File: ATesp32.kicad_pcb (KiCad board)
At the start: 4 copper layers, 18 x 51.2 mm, 51 parts, among them J1 USB_C_Receptacle_USB2.0_16P, J2 JST PH, Q1 DMP2045U, SW1 SW_Push, SW2 SW_Push, U1 ESP32-S3, U2 ATmega32A-P, U3 MCP73831-2-OT, U4 AP2112K-3.3, U5 CP2102N-Axx-xQFN24, Y1 40 MHz

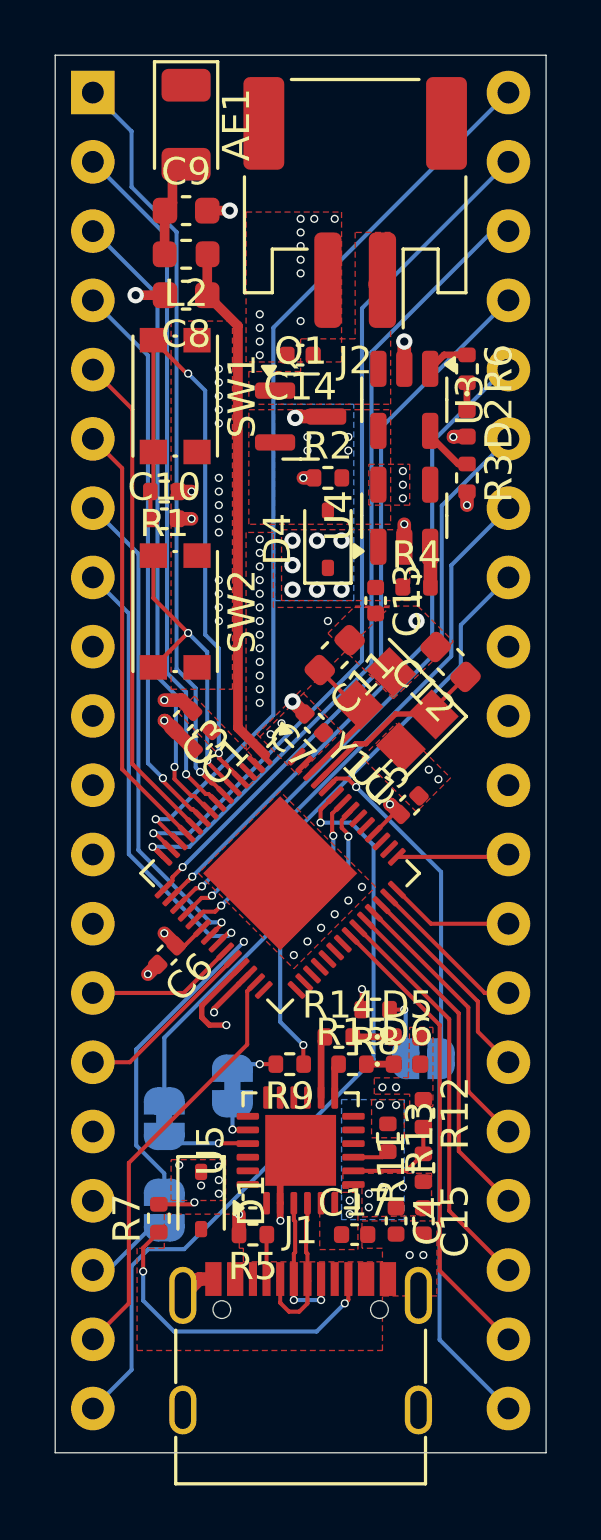
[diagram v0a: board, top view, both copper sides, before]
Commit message: cleanup
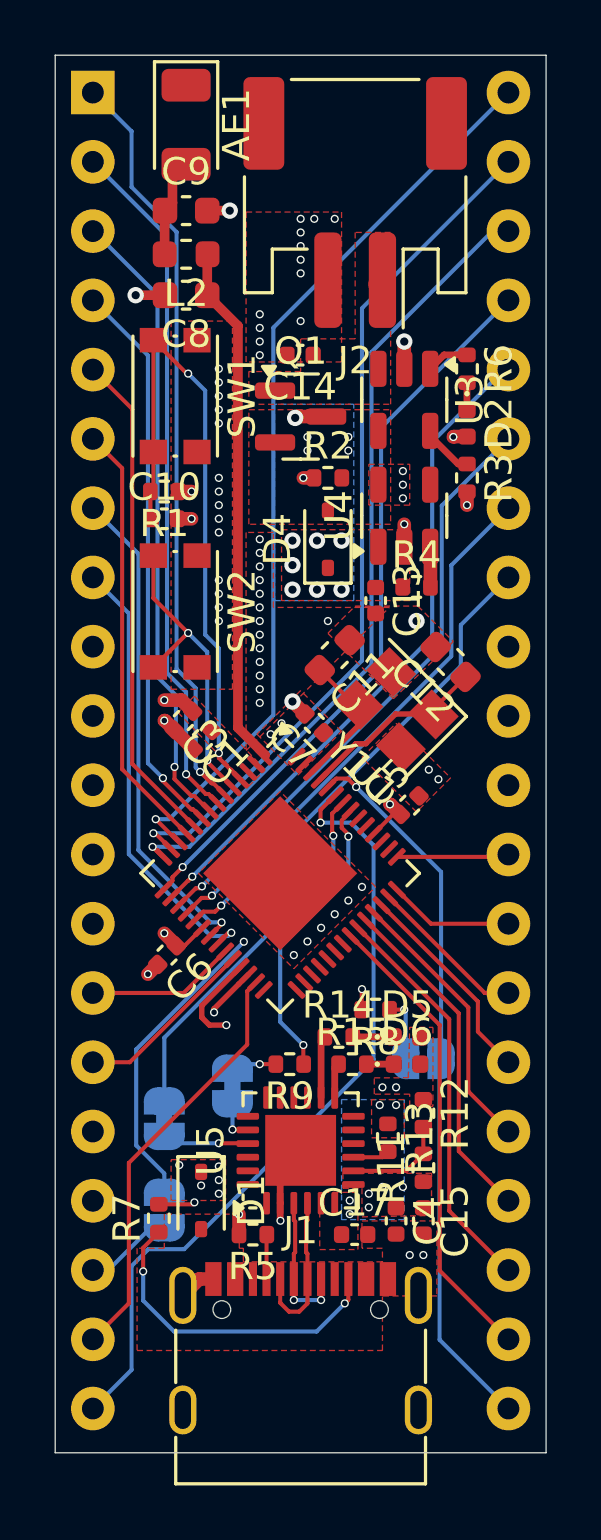
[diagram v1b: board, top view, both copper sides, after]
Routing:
- net GND: track 15.4 -> 14.3 mm
- net PD4: track 3.26 -> 2.19 mm
- net PA2: track 29.7 -> 29.1 mm
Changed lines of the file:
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@@
 	)
 	(segment
-		(start 79.0125 55.7125)
-		(end 79.025 55.7)
-		(width 0.355542)
-		(layer "F.Cu")
-		(net 1)
-	)
-	(segment
 		(start 79.8 54)
 		(end 79.3 54.5)
@@
 	)
 	(segment
-		(start 83.25 90.9125)
-		(end 84 90.1625)
-		(width 0.25)
-		(layer "F.Cu")
-		(net 3)
-	)
-	(segment
 		(start 83.25 92.1)
 		(end 83.25 92.732108)
@@
 	)
 	(segment
-		(start 80.5 55.775)
-		(end 80.525 55.75)
-		(width 0.355542)
-		(layer "F.Cu")
-		(net 3)
-	)
-	(segment
 		(start 80.28 94.88)
 		(end 79.68 95.48)
@@
 	)
 	(segment
-		(start 87.390488 77.839411)
-		(end 87.660589 77.839411)
-		(width 0.15)
-		(layer "F.Cu")
-		(net 5)
-	)
-	(segment
-		(start 79.439411 82.639411)
-		(end 79.439411 82.660589)
-		(width 0.5)
-		(layer "F.Cu")
-		(net 5)
-	)
-	(segment
 		(start 80.039411 74.060589)
 		(end 79.628822 73.65)
@@
 	)
 	(segment
-		(start 80.575 57.3125)
-		(end 80.5875 57.3)
-		(width 0.355542)
-		(layer "F.Cu")
-		(net 7)
-	)
-	(segment
 		(start 80.575 58.8)
 		(end 81.7 59.925)
@@
 	)
 	(segment
-		(start 78.6 65.890001)
-		(end 78.490001 66)
-		(width 0.15)
-		(layer "F.Cu")
-		(net 8)
-	)
-	(segment
-		(start 78.490001 66.970001)
-		(end 78.52 67)
-		(width 0.15)
-		(layer "F.Cu")
-		(net 8)
-	)
-	(segment
 		(start 78.6 60.45)
 		(end 78.6 64.55)
@@
 	)
 	(segment
-		(start 84.324991 94.954991)
-		(end 84.25 94.88)
-		(width 0.15)
-		(layer "F.Cu")
-		(net 16)
-	)
-	(segment
 		(start 84.25 93.949999)
 		(end 84.2 93.899999)
@@
 	)
 	(segment
-		(start 83.25 94.88)
-		(end 83.175 94.955)
-		(width 0.15)
-		(layer "F.Cu")
-		(net 16)
-	)
-	(segment
 		(start 84.25 95.775)
 		(end 84.25 94.88)
@@
 	)
 	(segment
-		(start 82.75 93.26)
-		(end 82.76 93.25)
-		(width 0.15)
-		(layer "F.Cu")
-		(net 18)
-	)
-	(segment
 		(start 82.75 94.88)
 		(end 82.75 93.26)
@@
 	)
 	(segment
-		(start 76.38 94.55)
-		(end 76.95 94.55)
-		(width 0.15)
-		(layer "B.Cu")
-		(net 21)
-	)
-	(segment
 		(start 76.95 94.55)
 		(end 78.5 93)
@@
 	)
 	(segment
-		(start 78.5 93)
-		(end 79 93)
-		(width 0.15)
-		(layer "B.Cu")
-		(net 21)
-	)
-	(segment
 		(start 78.6 69.9125)
 		(end 78.6 68.35)
@@
 		(net 26)
 	)
-	(segment
-		(start 82.05 89.9)
-		(end 82.0625 89.9125)
-		(width 0.15)
-		(layer "F.Cu")
-		(net 26)
-	)
 	(via
 		(at 81 89.9)
@@
 	)
 	(segment
-		(start 79.25 89.9)
-		(end 79 89.65)
-		(width 0.15)
-		(layer "B.Cu")
-		(net 26)
-	)
-	(segment
 		(start 81 89.9)
 		(end 79.25 89.9)
@@
 	)
 	(segment
-		(start 81.65 87)
-		(end 81.5 87.15)
-		(width 0.15)
-		(layer "B.Cu")
-		(net 27)
-	)
-	(segment
 		(start 81.5 89.4)
 		(end 82.05 89.4)
@@
 		(net 28)
 	)
-	(segment
-		(start 82.05 89.4)
-		(end 82.0625 89.4125)
-		(width 0.15)
-		(layer "F.Cu")
-		(net 28)
-	)
 	(via
 		(at 81.5 89.4)
@@
 	)
 	(segment
-		(start 88.75 63.963172)
-		(end 88.75 63.775)
-		(width 0.25)
-		(layer "F.Cu")
-		(net 29)
-	)
-	(segment
 		(start 88.76 69.5)
 		(end 88.76 68.035)
@@
 	)
 	(segment
-		(start 88.76 68.035)
-		(end 88.75 68.025)
-		(width 0.5)
-		(layer "F.Cu")
-		(net 30)
-	)
-	(segment
 		(start 85.50496 78.330518)
 		(end 85.50496 78.063238)
@@
 	)
 	(segment
-		(start 84.1 86.99)
-		(end 84.11 87)
-		(width 0.15)
-		(layer "F.Cu")
-		(net 31)
-	)
-	(segment
 		(start 85.75 78.575558)
 		(end 85.50496 78.330518)
@@
 	)
 	(segment
-		(start 85.83094 77.737258)
-		(end 85.83094 77.701903)
-		(width 0.15)
-		(layer "F.Cu")
-		(net 31)
-	)
-	(segment
 		(start 84.1 86.3)
 		(end 84.1 86.99)
@@
 	)
 	(segment
-		(start 84.75 86.14)
-		(end 84.89 86)
-		(width 0.25)
-		(layer "F.Cu")
-		(net 34)
-	)
-	(segment
 		(start 84.75 88.225)
 		(end 84.75 86.14)
@@
 	)
 	(segment
-		(start 85.25 87.14)
-		(end 85.39 87)
-		(width 0.25)
-		(layer "F.Cu")
-		(net 35)
-	)
-	(segment
 		(start 85.25 88.225)
 		(end 85.25 87.14)
@@
 	)
 	(segment
-		(start 78.972004 79.398959)
-		(end 78.936647 79.398959)
-		(width 0.15)
-		(layer "F.Cu")
-		(net 36)
-	)
-	(segment
 		(start 78.936647 79.398959)
 		(end 78.568844 79.031156)
@@
 	)
 	(segment
-		(start 91.036827 56.45)
-		(end 91.62 56.45)
-		(width 0.15)
-		(layer "B.Cu")
-		(net 36)
-	)
-	(segment
 		(start 86.6 72.349098)
 		(end 86.6 60.886827)
@@
 	)
 	(segment
-		(start 80.636898 77.701903)
-		(end 80.66906 77.701903)
-		(width 0.15)
-		(layer "F.Cu")
-		(net 38)
-	)
-	(segment
 		(start 79.990524 77.161596)
 		(end 80.096591 77.161596)
@@
 	)
 	(segment
-		(start 76.413173 56.45)
-		(end 76.38 56.45)
-		(width 0.15)
-		(layer "B.Cu")
-		(net 38)
-	)
-	(segment
 		(start 78.75 72.798959)
 		(end 78.75 58.786827)
@@
 	)
 	(segment
-		(start 91.531041 79.398959)
-		(end 91.62 79.31)
-		(width 0.15)
-		(layer "F.Cu")
-		(net 43)
-	)
-	(segment
 		(start 78.670867 78.532137)
 		(end 79.254847 79.116117)
@@
 	)
 	(segment
-		(start 91.62 61.53)
-		(end 91.468959 61.53)
-		(width 0.15)
-		(layer "B.Cu")
-		(net 46)
-	)
-	(segment
 		(start 91.468959 61.53)
 		(end 88.825 64.173959)
@@
 	)
 	(segment
-		(start 76.38 89.380228)
-		(end 76.38 89.47)
-		(width 0.15)
-		(layer "B.Cu")
-		(net 69)
-	)
-	(segment
-		(start 79.502334 78.833274)
-		(end 79.537689 78.833274)
-		(width 0.15)
-		(layer "F.Cu")
-		(net 70)
-	)
-	(segment
 		(start 78.68453 78.01547)
 		(end 79.502334 78.833274)
@@
 	)
 	(segment
-		(start 85.977207 73.823223)
-		(end 86.121142 73.823223)
-		(width 0.15)
-		(layer "F.Cu")
-		(net 92)
-	)
-	(segment
 		(start 88.8617 74.159619)
 		(end 87.4818 74.159619)
@@
 	)
 	(segment
-		(start 88.878858 73.967158)
-		(end 88.878858 74.176777)
-		(width 0.15)
-		(layer "F.Cu")
-		(net 93)
-	)
-	(segment
 		(start 86.020101 75.25)
 		(end 84.699569 76.570532)
 		(width 0.2)
 		(layer "F.Cu")
-		(net 93)
-	)
-	(segment
-		(start 88.878858 74.176777)
-		(end 88.8617 74.159619)
-		(width 0.2)
-		(layer "F.Cu")

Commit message: fix silk
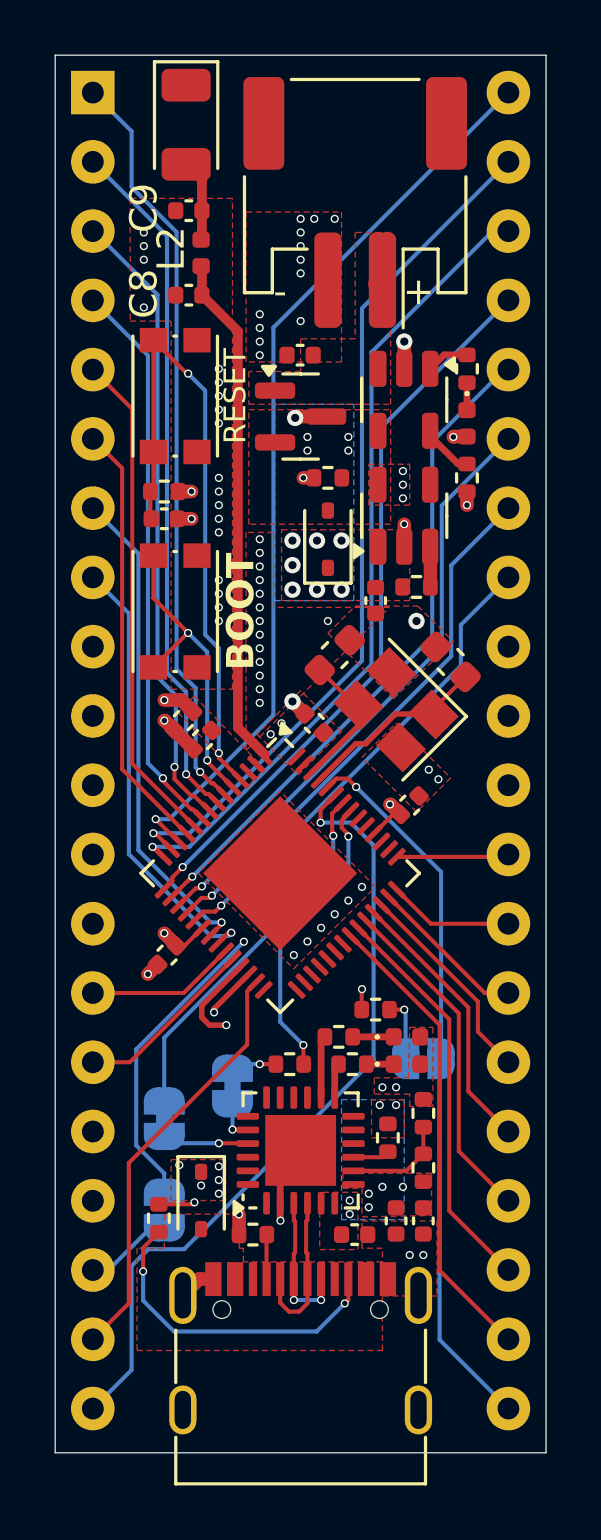
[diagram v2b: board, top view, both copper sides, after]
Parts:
- C8, C9: footprint Capacitor_SMD:C_0603_1608Metric -> Capacitor_SMD:C_0402_1005Metric
- L2: footprint Inductor_SMD:L_0603_1608Metric -> Inductor_SMD:L_0402_1005Metric
- SW1: value SW_Push -> RESET
- SW2: value SW_Push -> BOOT
- moved L2 0.55 mm to (80.3, 57.2), turned to 90 degrees
- moved C8 0.10 mm to (79.9, 58.8)
- moved C9 0.10 mm to (79.9, 55.7), turned to 180 degrees
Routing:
- net GND: track 14.3 -> 12.4 mm, vias 68 -> 70
- net Net-(AE1-PCB_Trace): track 3.61 -> 3.02 mm
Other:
- board text added: "+"
- board text added: "-"
